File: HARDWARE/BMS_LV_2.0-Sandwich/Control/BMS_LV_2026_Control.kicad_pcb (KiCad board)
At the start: 6 copper layers, 62.5 x 40.8 mm, 104 parts, among them IC1 TAR5S33UTE85LF, IC2 TAR5S33UTE85LF, IC4 TPS54202HDDCR, J1 Conn_01x26, J3 FTSH-107-01-L-D-K, J6 Conn_01x09_Female, U1 STM32G484RETx, U7 ADM3057ExRW, Y1 ATX-11-F-32.000MHZ-F05-T

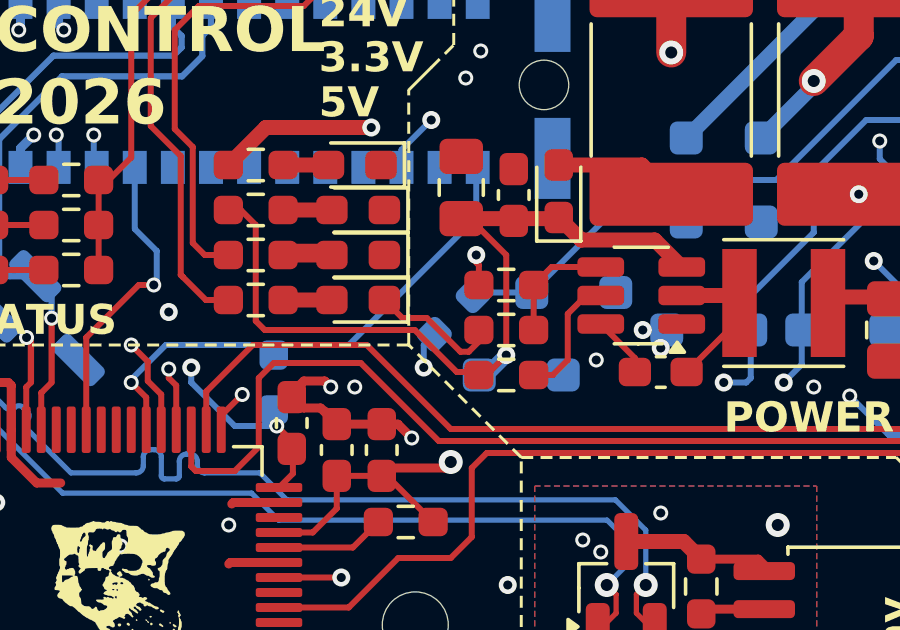
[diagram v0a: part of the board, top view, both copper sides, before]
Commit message: Gotowe do review
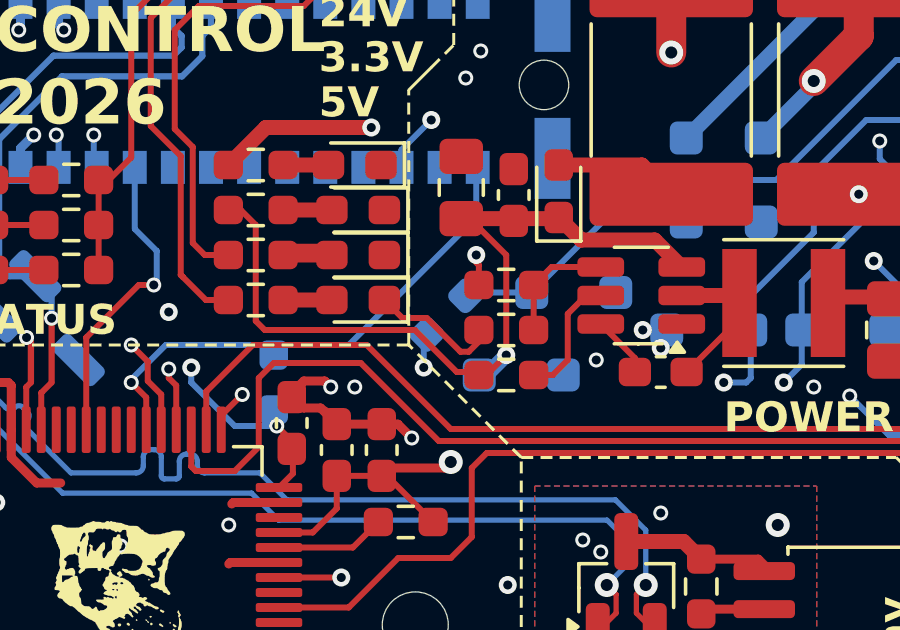
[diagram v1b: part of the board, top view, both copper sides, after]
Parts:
- moved R29 0.25 mm to (162.8, 93.0)
